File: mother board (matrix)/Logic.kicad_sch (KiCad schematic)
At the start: 1 part, among them U1 STM32F030C6Tx

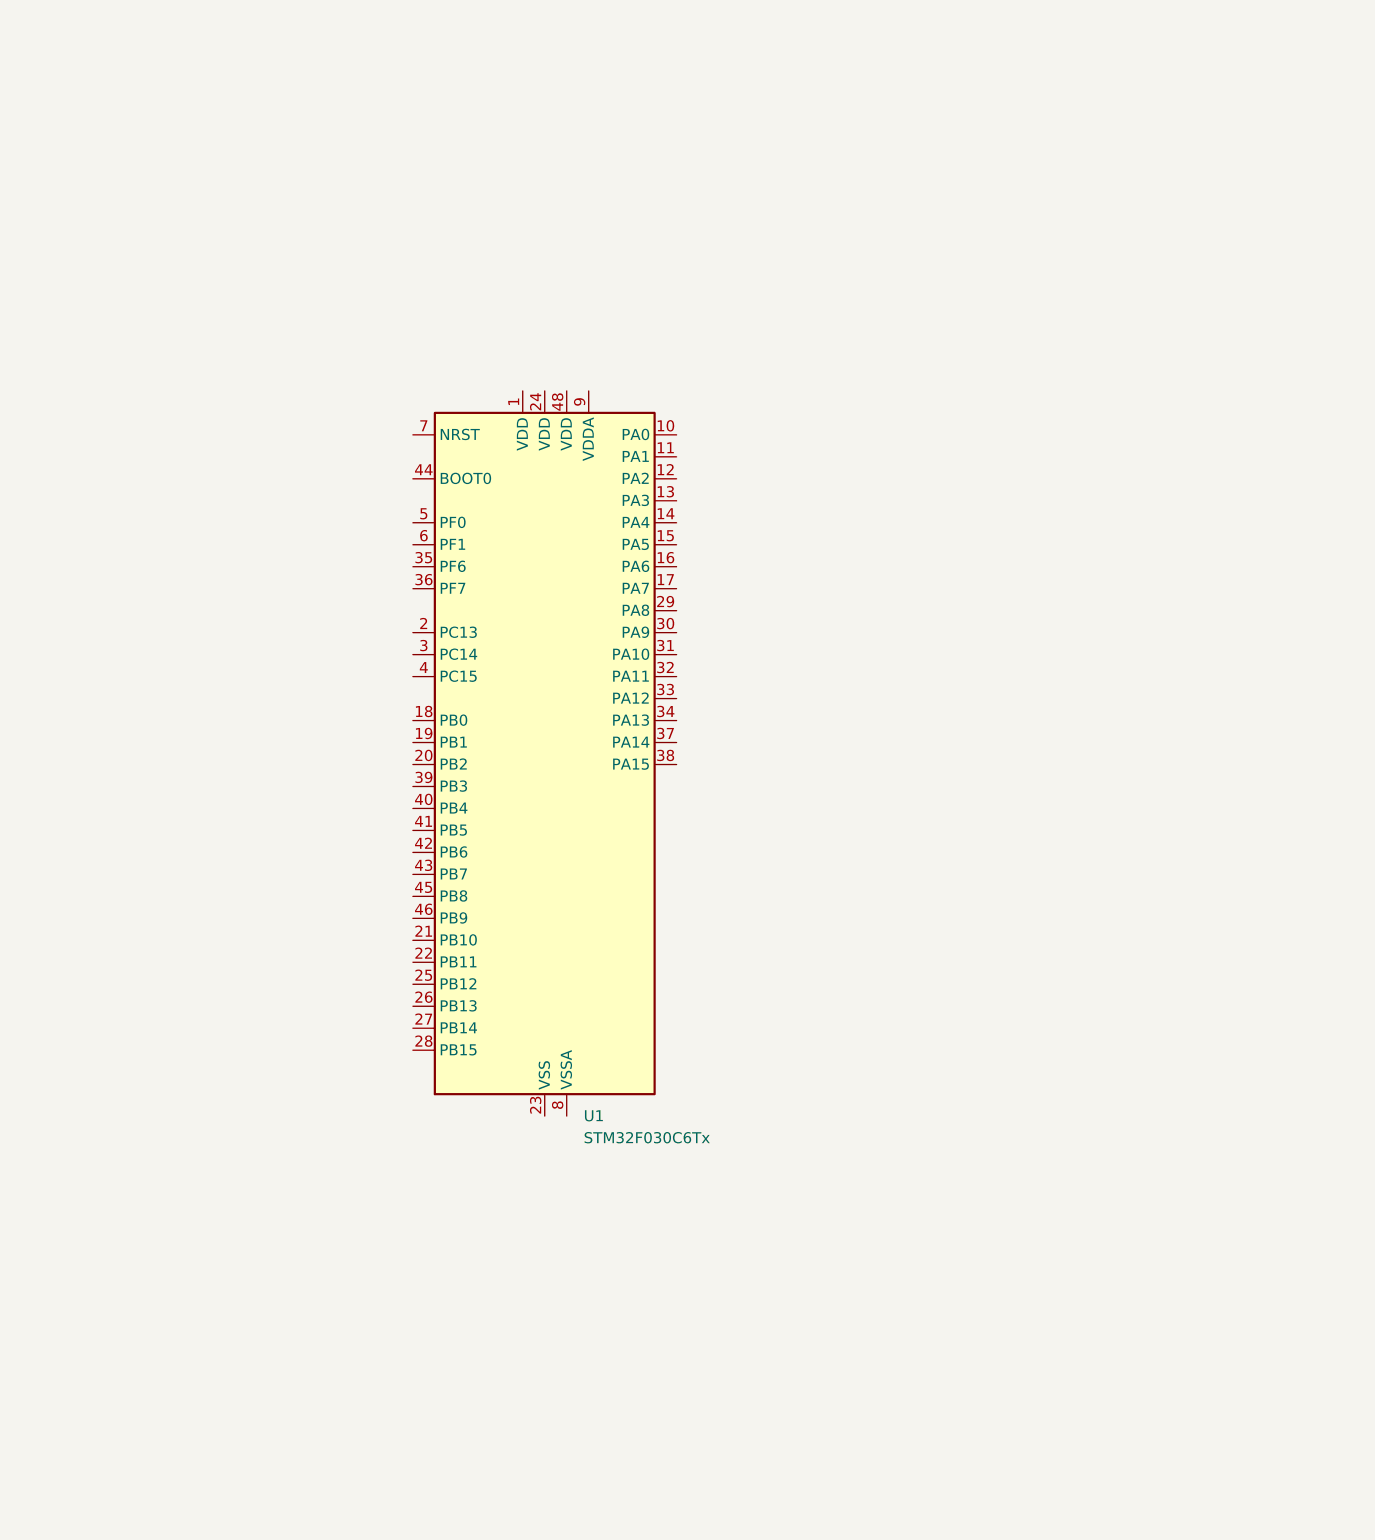
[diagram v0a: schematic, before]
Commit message: changes
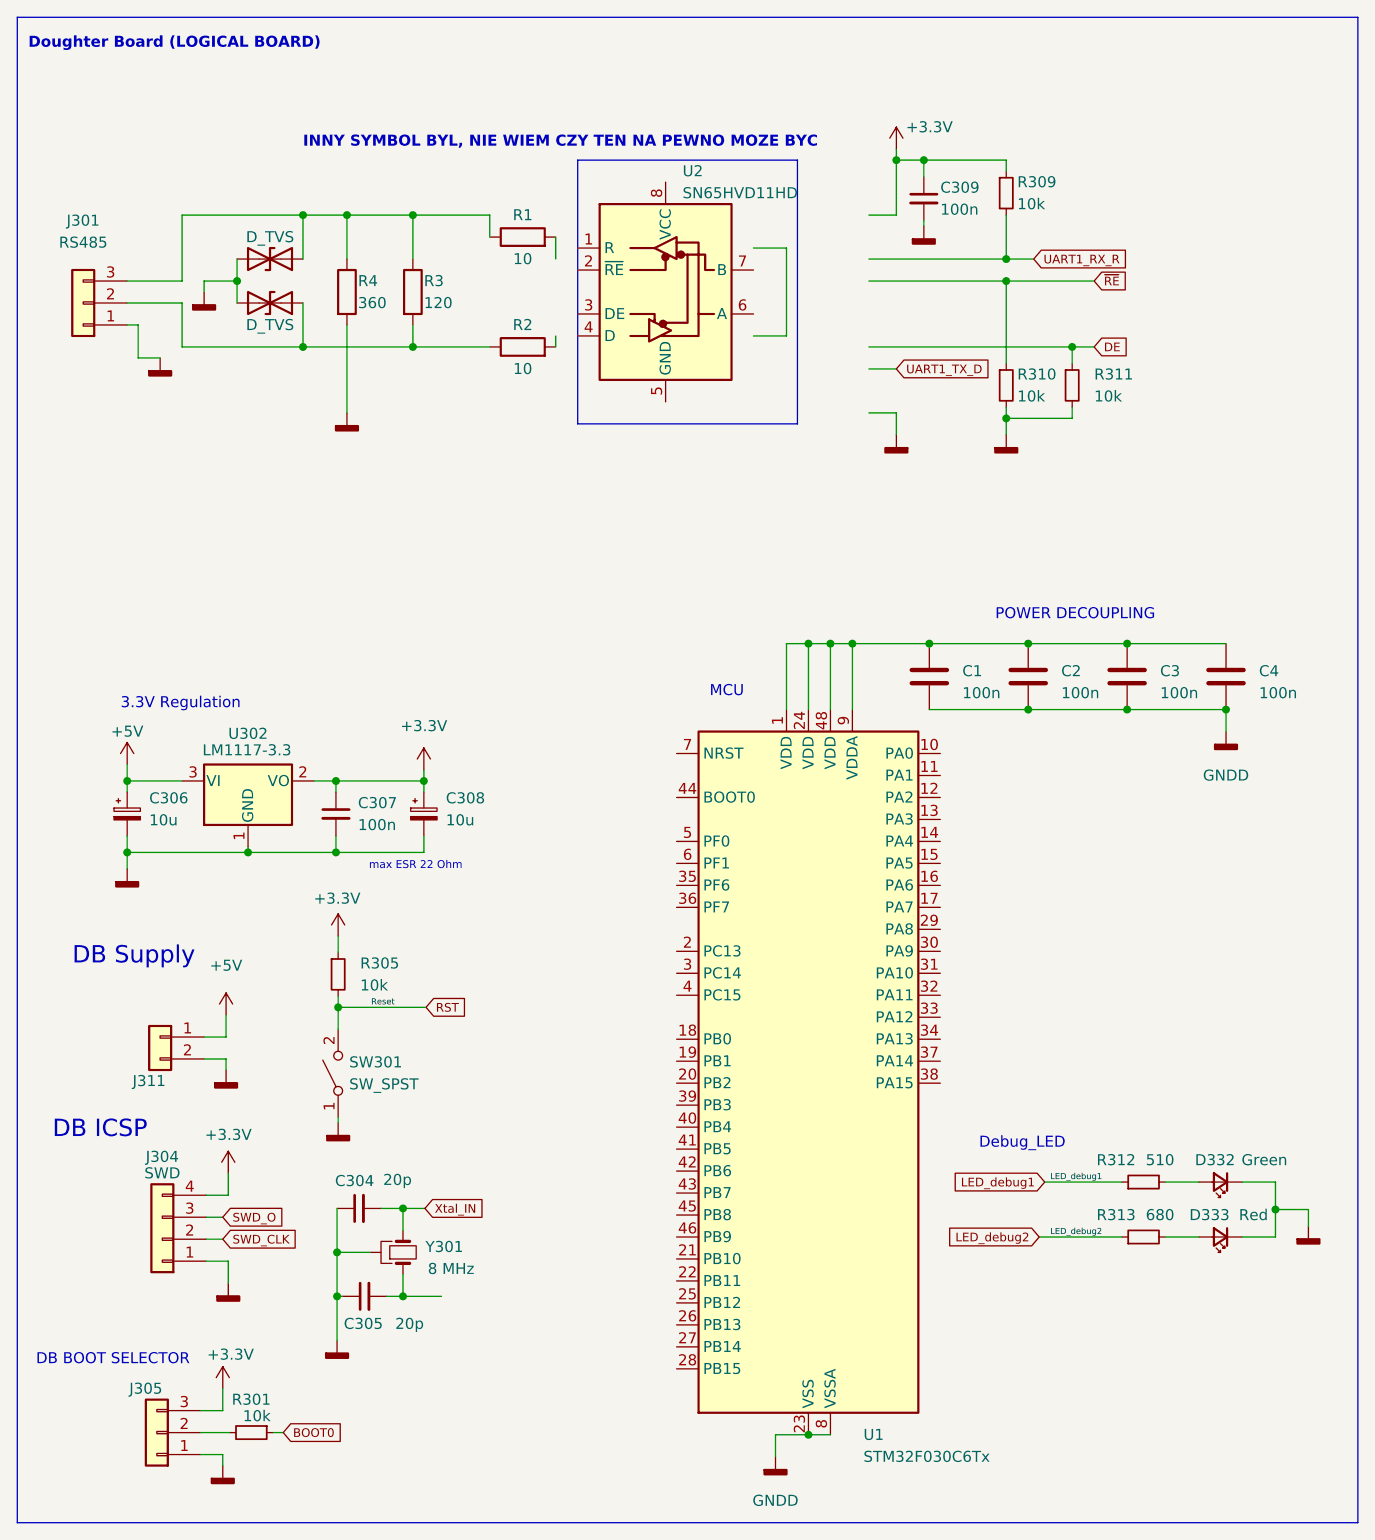
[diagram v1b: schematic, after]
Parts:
- added C1, C2, C3, C4: 100n, symbol Device:C
- added C304, C305: 20p, Capacitor_SMD:C_0603_1608Metric_Pad1.08x0.95mm_HandSolder, symbol Device:C_Small
- added C306, C308: 10u, Capacitor_Tantalum_SMD:CP_EIA-6032-28_Kemet-C_Pad2.25x2.35mm_HandSolder, symbol Device:C_Polarized_Small
- added C307, C309: 100n, Capacitor_SMD:C_0603_1608Metric_Pad1.08x0.95mm_HandSolder, symbol Device:C_Small
- added D1, D2: D_TVS, symbol Device:D_TVS
- added D332: Green, LED_SMD:LED_0805_2012Metric_Pad1.15x1.40mm_HandSolder, symbol Device:LED_Small
- added D333: Red, LED_SMD:LED_0805_2012Metric_Pad1.15x1.40mm_HandSolder, symbol Device:LED_Small
- added J301: RS485, Connector_PinSocket_2.54mm:PinSocket_1x03_P2.54mm_Vertical_SMD_Pin1Right, symbol Connector_Generic:Conn_01x03
- added J304: SWD, Connector_PinSocket_2.54mm:PinSocket_1x04_P2.54mm_Vertical_SMD_Pin1Right, symbol Connector_Generic:Conn_01x04
- added J305: BOOT_TO/ SELECTOR, Connector_PinHeader_2.54mm:PinHeader_1x03_P2.54mm_Vertical_SMD_Pin1Left, symbol Connector_Generic:Conn_01x03
- added J311: BOOT_TO/ SELECTOR, Connector_PinHeader_2.54mm:PinHeader_1x02_P2.54mm_Vertical_SMD_Pin1Left, symbol Connector_Generic:Conn_01x02
- added R1, R2: 10, symbol Device:R
- added R3: 120, symbol Device:R
- added R301, R305, R309, R310, R311: 10k, Resistor_SMD:R_0603_1608Metric_Pad0.98x0.95mm_HandSolder, symbol Device:R_Small
- added R312: 510, Resistor_SMD:R_0603_1608Metric_Pad0.98x0.95mm_HandSolder, symbol Device:R_Small
- added R313: 680, Resistor_SMD:R_0603_1608Metric_Pad0.98x0.95mm_HandSolder, symbol Device:R_Small
- added R4: 360, symbol Device:R
- added SW301: SW_SPST, Button_Switch_SMD:SW_SPST_EVQPE1, symbol Switch:SW_SPST
- added U2: SN65HVD11HD, Package_SO:SOIC-8_3.9x4.9mm_P1.27mm, symbol Interface_UART:SN65HVD11HD
- added U302: LM1117-3.3, Package_TO_SOT_SMD:SOT-223, symbol Regulator_Linear:LM1117-3.3
- added Y301: 8 MHz, Crystal:Crystal_SMD_Abracon_ABM3C-4Pin_5.0x3.2mm, symbol Device:Crystal_Small
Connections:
- net at U1.1 (VDD): now also U1.24 (VDD), U1.48 (VDD), U1.9 (VDDA), C1.1, C2.1, C3.1, C4.1
- net GNDD: now reaches U1.23 (VSS), U1.47 (VSS)
- net GNDD: now also U1.8 (VSSA), C1.2, C2.2, C3.2, C304.1, C305.1, C306.2, C307.2, C308.2, C309.2, C4.2, D1.2 (A2), D2.2 (A2), D332.1 (K), D333.1 (K), J301.1 (Pin_1), J304.1 (Pin_1), J305.1 (Pin_1), J311.2 (Pin_2), R310.2, R311.2, R4.2, SW301.1 (A), U302.1 (GND), Y301.2 (GND), Y301.4 (GND)
- new net: C305.2, Y301.1
- new net: D1.1 (A1), J301.3 (Pin_3), R1.1, R3.1, R4.1
- new net: D2.1 (A1), J301.2 (Pin_2), R2.1, R3.2
- new net: J305.2 (Pin_2), R301.2
- new net: D333.2 (A), R313.2
- new net: D332.2 (A), R312.2
- new net +3.3V: C307.1, C308.1, C309.1, J304.4 (Pin_4), J305.3 (Pin_3), R305.1, R309.1, U302.2 (VO), U302.4 (VO)
- new net +5V: C306.1, J311.1 (Pin_1), U302.3 (VI)
- new net BOOT0: R301.1
- new net DE: R311.1
- new net LED_debug1: R312.1
- new net LED_debug2: R313.1
- new net RST: R305.2, SW301.2 (B)
- new net SWD_CLK: J304.2 (Pin_2)
- new net SWD_O: J304.3 (Pin_3)
- new net UART1_RX_R: R309.2
- new net Xtal_IN: C304.2, Y301.3
- new net ~{RE}: R310.1
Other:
- note added: "3.3V Regulation"
- note added: "DB BOOT SELECTOR"
- note added: "DB ICSP"
- note added: "DB Supply"
- note added: "Debug_LED"
- note added: "Doughter Board (LOGICAL BOARD)"
- note added: "INNY SYMBOL BYL, NIE WIEM CZY TEN NA PEWNO MOZE BYC"
- note added: "MCU"
- note added: "POWER DECOUPLING"
- note added: "max ESR 22 Ohm"
- moved on the sheet: U1
